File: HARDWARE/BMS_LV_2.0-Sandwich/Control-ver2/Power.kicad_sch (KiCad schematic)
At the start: 25 parts, among them IC1 TAR5S33UTE85LF, IC4 TPS54202HDDCR

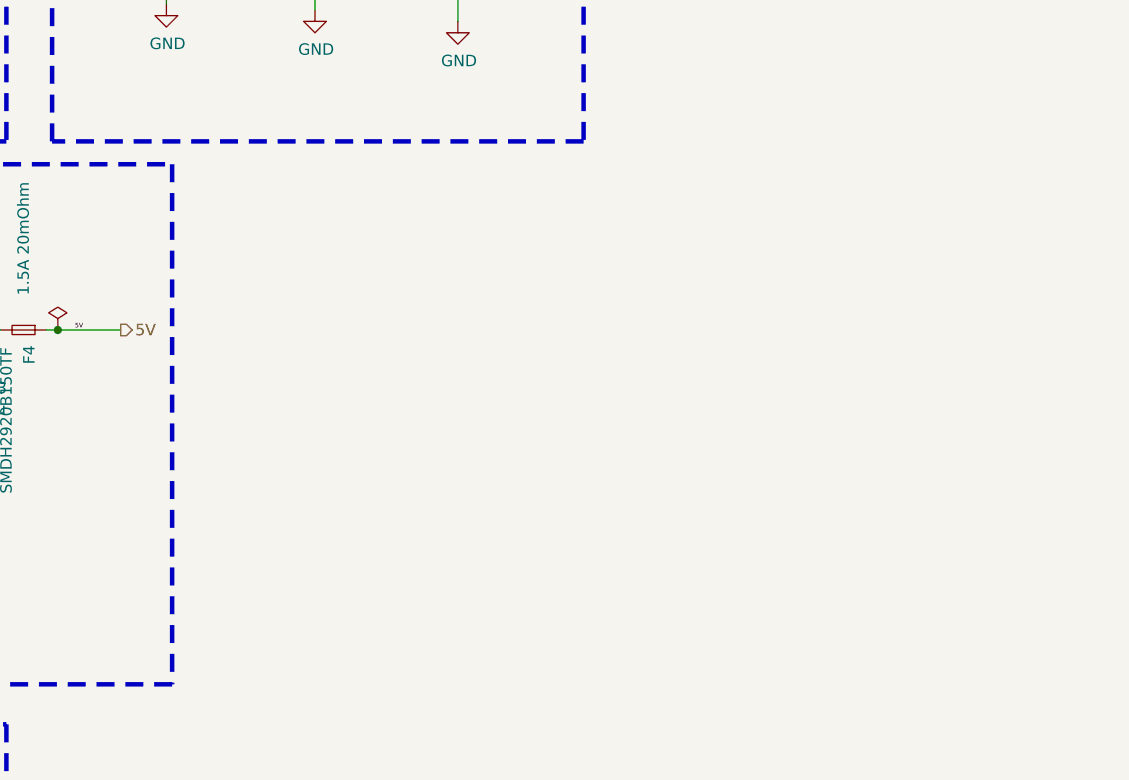
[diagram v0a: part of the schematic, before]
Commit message: Kolejna kurwa wersja gotowa, japierdole
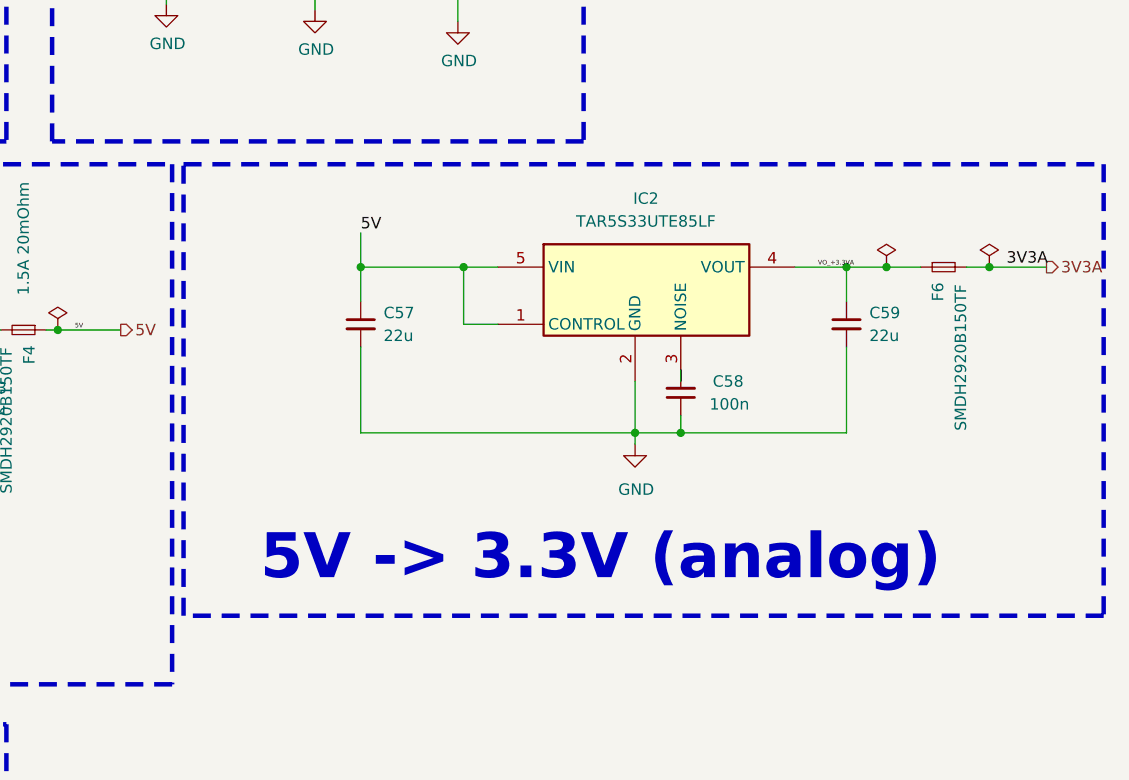
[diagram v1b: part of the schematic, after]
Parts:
- added C57, C59: 22u, Capacitor_SMD:C_0805_2012Metric_Pad1.18x1.45mm_HandSolder, symbol Device:C_Small
- added C58: 100n, Capacitor_SMD:C_0603_1608Metric, symbol Device:C_Small
- added F6: SMDH2920B150TF, Fuse:Fuse_2920_7451Metric_Pad2.10x5.45mm_HandSolder, symbol Device:Fuse_Small
- added IC2: TAR5S33UTE85LF, Footprint:SOTFL65P210X75-5N, symbol TAR5S33UTE85LF:TAR5S33UTE85LF
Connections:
- net 5V: now also C57.1, IC2.1 (CONTROL), IC2.5 (VIN)
- net GND: now also C57.2, C58.1, C59.2, IC2.2 (GND)
- new net: C58.2, IC2.3 (NOISE)
- new net 3V3A: F6.2
- new net VO_+3.3VA: C59.1, F6.1, IC2.4 (VOUT)
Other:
- note added: "5V -> 3.3V (analog)"
